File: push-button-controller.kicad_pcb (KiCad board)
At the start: 2 copper layers, 96.9 x 89.5 mm, 90 parts, among them J1 Conn_01x04, J10 Conn_01x02, J11 Conn_01x04, J12 Conn_01x02, J2 Conn_01x02, J3 Conn_01x02, J4 Conn_01x04, J5 Conn_01x02, J6 Conn_01x02, J7 Conn_01x04, J8 Conn_01x02, J9 Conn_01x02, SW1 SW_Push, SW2 SW_Push, SW3 SW_Push, SW4 SW_Push, U1 LTC2954CTS8-2_TRPBF, U2 LTC2950ITS8-2_TRMPBF, U3 LTC2951ITS8-1, U4 LTC2955CTS8-2_TRPBF

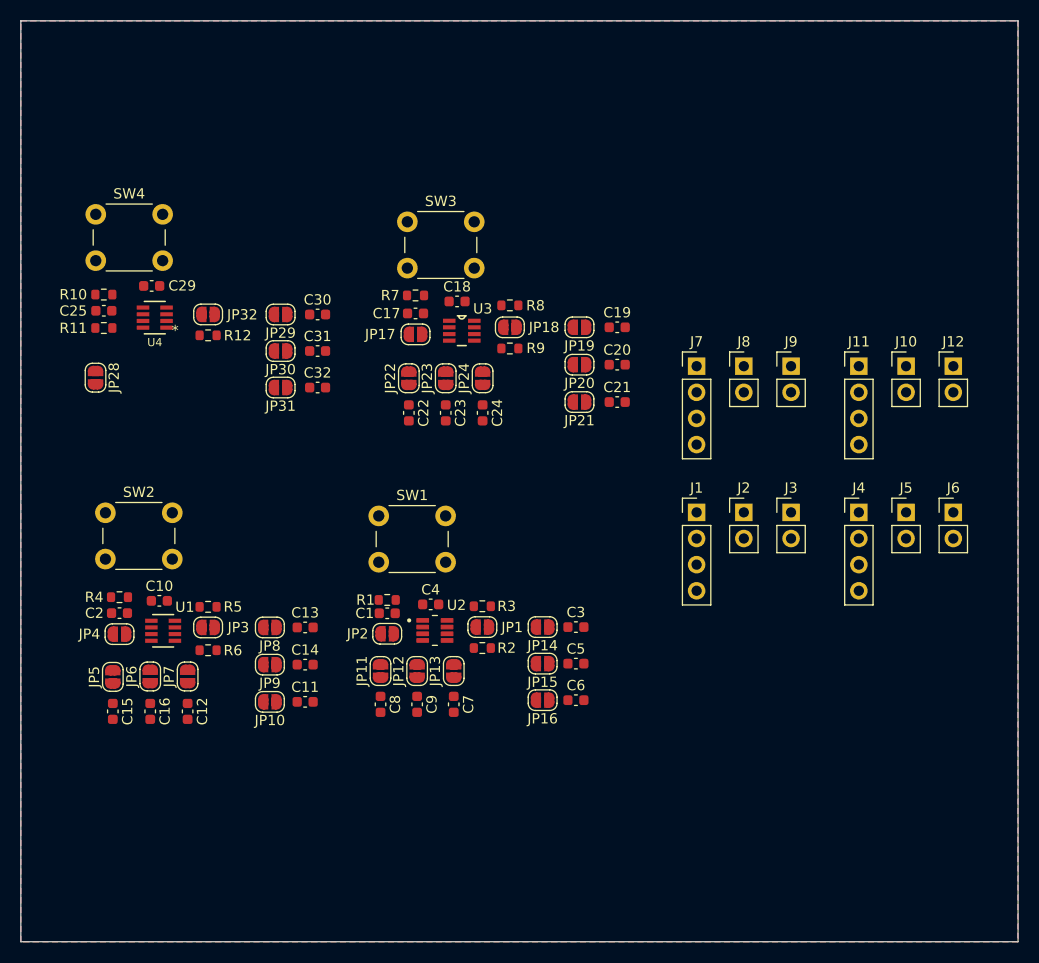
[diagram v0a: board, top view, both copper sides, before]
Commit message: Finished, 1st PCB order to JLCPCB
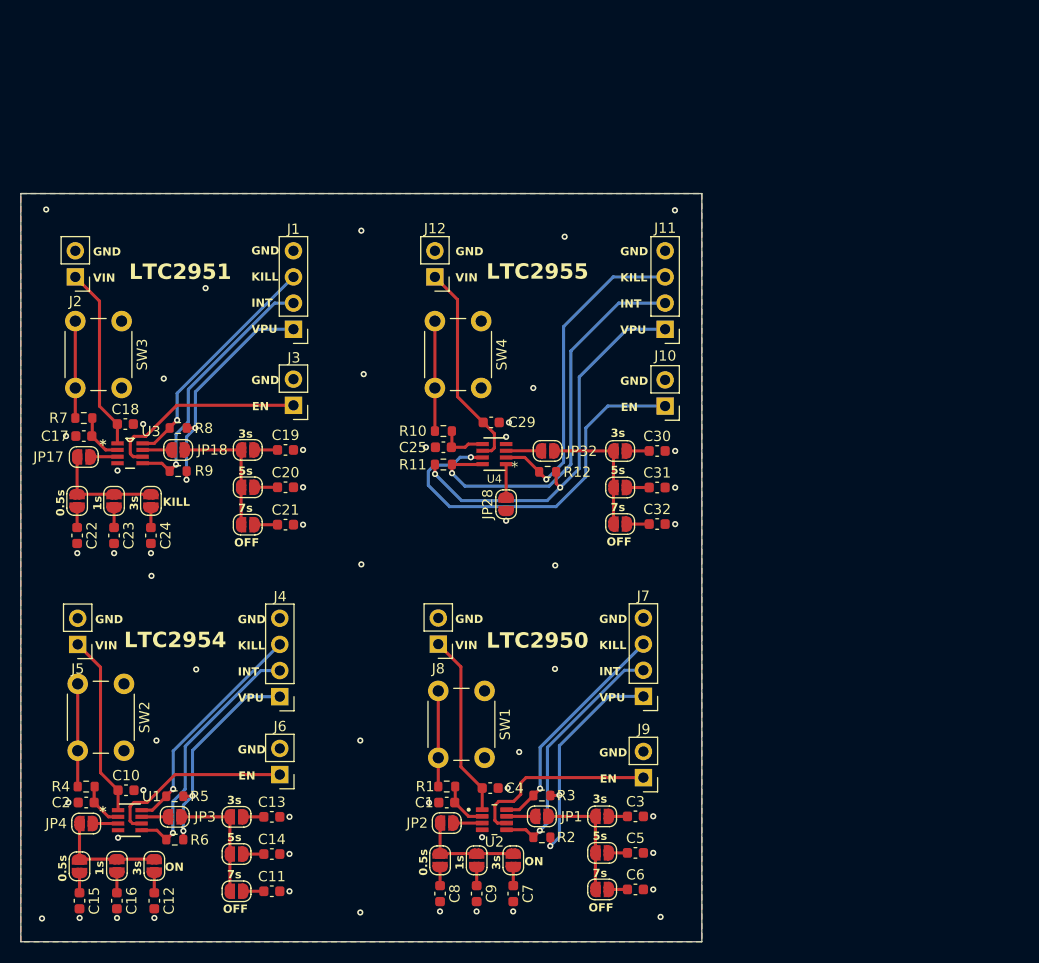
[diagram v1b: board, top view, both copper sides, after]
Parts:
- C12: value 320 -> 470nF
- C14, C20, C5: value 780nF -> 820nF
- C15, C22, C8: value 78nF -> 82nF
- C16, C23, C9: value 160nF -> 150nF
- C32: value 1.2uF -> 1.5uF
- C7: value 320nF -> 330nF
- moved J5 81.5 mm to (105.2, 110.5), turned to 180 degrees
- moved J6 70.2 mm to (124.8, 123.2), turned to 180 degrees
- moved J2 68.9 mm to (105.0, 74.8), turned to 180 degrees
- moved J4 59.1 mm to (124.8, 115.6), turned to 180 degrees
- moved J12 51.1 mm to (139.9, 74.8), turned to 180 degrees
- moved J3 49.5 mm to (126.2, 87.3), turned to 180 degrees
- moved J1 43.0 mm to (126.2, 79.9), turned to 180 degrees
- moved J9 42.5 mm to (160.2, 123.5), turned to 180 degrees
- moved JP28 41.8 mm to (146.8, 96.9), turned to 90 degrees
- moved J8 40.2 mm to (140.2, 110.5), turned to 180 degrees
- moved SW4 38.9 mm to (144.4, 79.1), turned to -90 degrees
- moved C29 35.6 mm to (145.4, 88.9)
- moved JP29 35.6 mm to (157.9, 91.7)
- moved JP30 35.6 mm to (157.9, 95.3)
- moved JP31 35.6 mm to (157.9, 98.8)
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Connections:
- C10 pad 1: VIN -> VIN_2954
- C18 pad 1: VIN -> VIN_2951
- C4 pad 1: VIN -> VIN_2950
- J1 pad 1: VPU -> VPU_2951
- J2 pad 1: VIN -> VIN_2951
- J4 pad 1: VPU -> VPU_2954
- J5 pad 1: VIN -> VIN_2954
- J7 pad 1: VPU -> VPU_2950
- J8 pad 1: VIN -> VIN_2950
- R2 pad 2: VPU -> VPU_2950
- R3 pad 2: VPU -> VPU_2950
- R5 pad 2: VPU -> VPU_2954
- R6 pad 2: VPU -> VPU_2954
- R8 pad 2: VPU -> VPU_2951
- R9 pad 2: VPU -> VPU_2951
- U1 pad 1: VIN -> VIN_2954
- U2 pad 1: VIN -> VIN_2950
- U3 pad 1: VIN -> VIN_2951
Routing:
- net /LTC2955/*INT: track 0.00 -> 38.9 mm, vias 0 -> 1
- net VPU: track 0.00 -> 38.2 mm, vias 0 -> 2
- net /LTC2955/EN/~{EN}: track 0.00 -> 37.9 mm, vias 0 -> 1
- net /LTC2955/*KILL: track 0.00 -> 32.2 mm, vias 0 -> 1
- net /LTC2951/~INT: track 0.00 -> 25.3 mm, vias 0 -> 1
- net /LTC2954/*INT: track 0.00 -> 24.9 mm, vias 0 -> 1
- net /LTC2950/~{INT}: track 0.00 -> 24.7 mm, vias 0 -> 1
- net /LTC2951/~KILL: track 0.00 -> 22.9 mm, vias 0 -> 1
- net VPU_2951: track 0.00 -> 22.6 mm, vias 0 -> 2
- net /LTC2950/~{KILL}: track 0.00 -> 22.3 mm, vias 0 -> 1
- net /LTC2954/*KILL: track 0.00 -> 22.3 mm, vias 0 -> 1
- net VPU_2950: track 0.00 -> 22.0 mm, vias 0 -> 2
- net VPU_2954: track 0.00 -> 20.6 mm, vias 0 -> 2
- net VIN: track 0.00 -> 20.3 mm
- net /LTC2951/EN/~{EN}: track 0.00 -> 19.9 mm
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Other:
- board size 96.9 x 89.5 mm -> 66.2 x 72.7 mm
- board text added: "*"
- board text added: "0.5s"
- board text added: "1s"
- board text added: "3s"
- board text added: "5s"
- board text added: "7s"
- board text added: "EN"
- board text added: "GND"
- board text added: "INT"
- board text added: "KILL"
- board text added: "LTC2950"
- board text added: "LTC2951"
- board text added: "LTC2954"
- board text added: "LTC2955"
- board text added: "OFF"
- board text added: "ON"
- board text added: "VIN"
- board text added: "VPU"
